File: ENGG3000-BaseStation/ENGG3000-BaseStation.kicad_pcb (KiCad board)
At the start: 4 copper layers, 79 x 43 mm, 57 parts, among them J1 OLED, J10 Cell/Pack 1, J2 Buttons, J3 UltrasonicA, J4 UltrasonicB, J5 USB_C_Receptacle_USB2.0_16P, J7 Power Switch, J8 Cell 3, J9 Cell 2, Q1 SS8050, Q2 AO3401A, SW1 RESET, SW2 BOOT, U1 ESP32-S3-WROOM-1-N16R8, U2 TPS63001DRCR, U3 CN3085

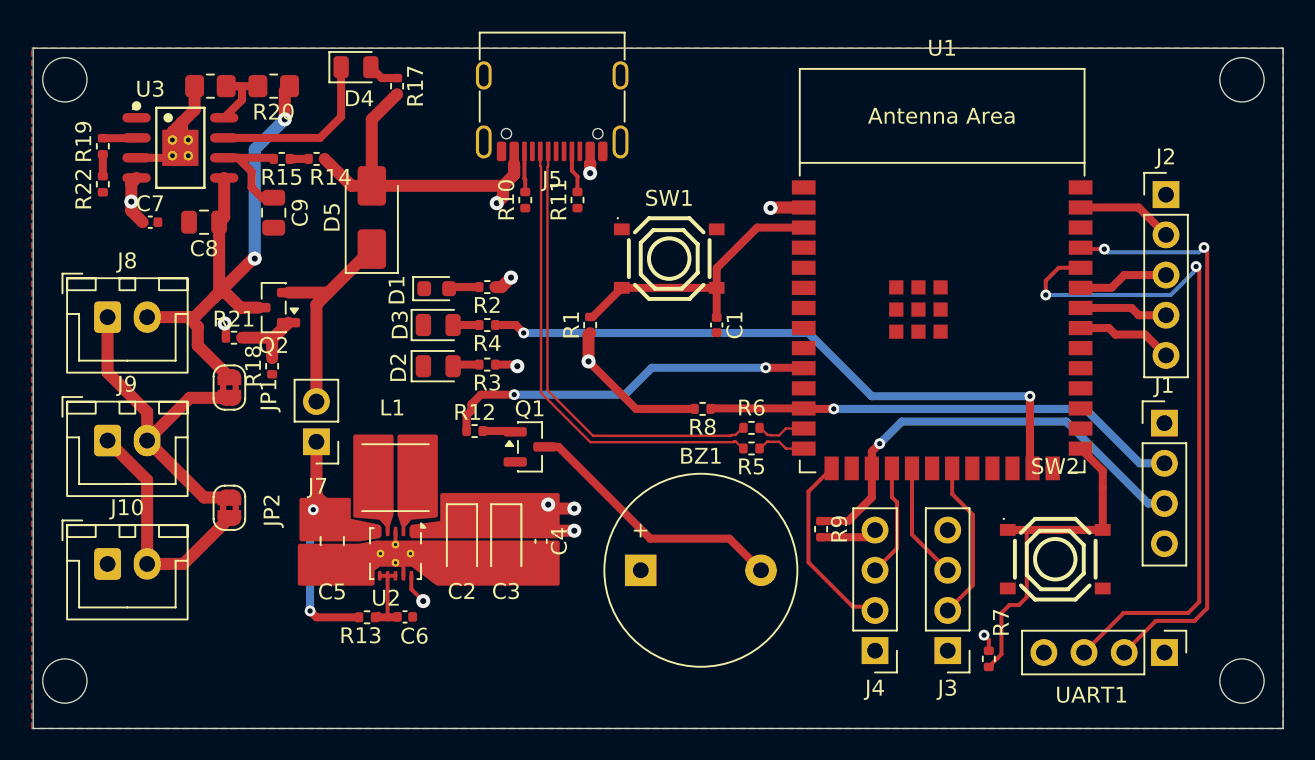
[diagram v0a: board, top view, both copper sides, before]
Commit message: Production ready PCB
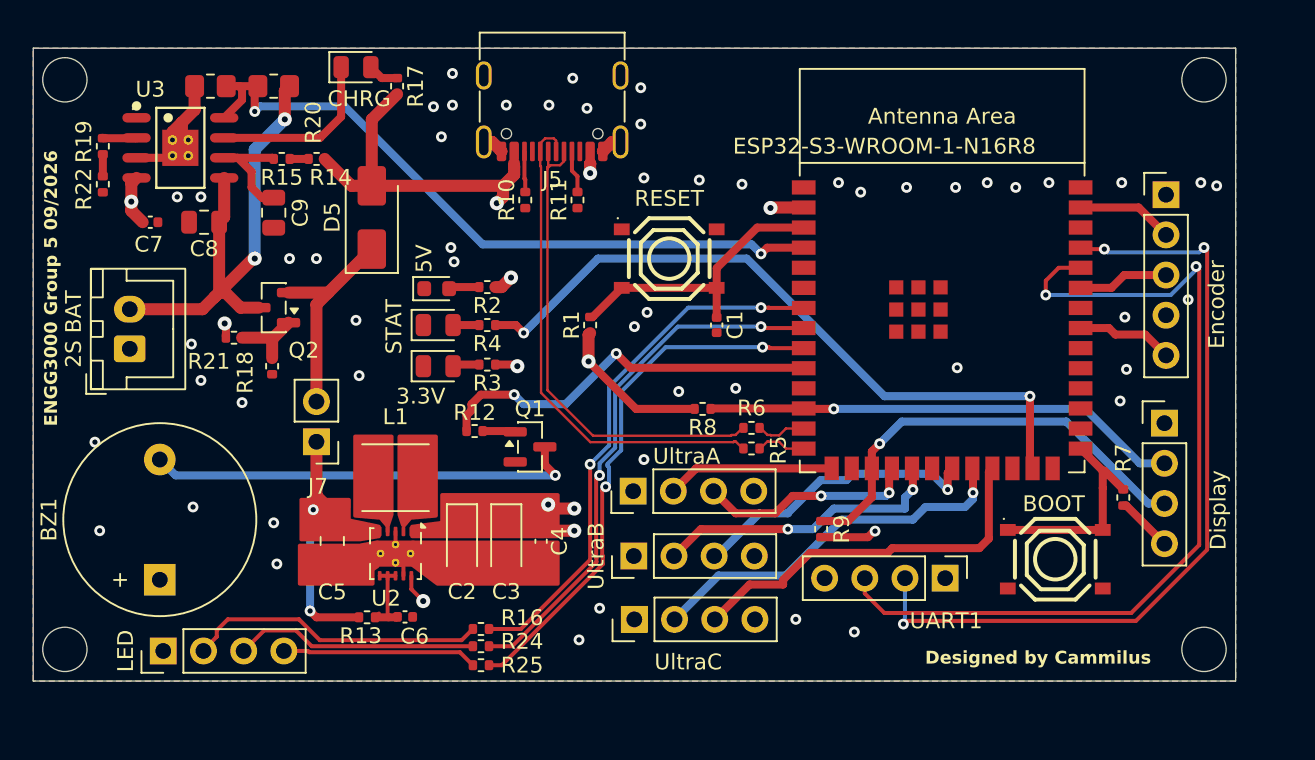
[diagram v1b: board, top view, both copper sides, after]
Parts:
- removed J8: Cell 3, Connector_JST:JST_XH_B2B-XH-A_1x02_P2.50mm_Vertical
- removed J9: Cell 2, Connector_JST:JST_XH_B2B-XH-A_1x02_P2.50mm_Vertical
- removed JP1, JP2: SolderJumper, Jumper:SolderJumper-2_P1.3mm_Bridged2Bar_RoundedPad1.0x1.5mm
- added G***: LOGO, LOGO, B.Cu at (136.5, 79.5)
- added G***: LOGO, LOGO, B.Cu at (167.8, 80.9)
- added LED: RGB LED, Connector_PinHeader_2.54mm:PinHeader_1x04_P2.54mm_Vertical, F.Cu at (118.2, 98.1)
- added R16: 330R, Resistor_SMD:R_0402_1005Metric, F.Cu at (138.3, 96.7)
- added R24: 220R, Resistor_SMD:R_0402_1005Metric, F.Cu at (138.3, 97.8)
- added R25: 220R, Resistor_SMD:R_0402_1005Metric, F.Cu at (138.3, 99.0)
- added UltraC: UltrasonicC, Connector_PinHeader_2.54mm:PinHeader_1x04_P2.54mm_Vertical, F.Cu at (148.0, 96.1)
- 2S BAT: renamed from J10; value Cell/Pack 1 -> NiMH 2S Pack
- Encoder: renamed from J2; value Buttons -> Encoder
- moved BZ1 30.4 mm to (118.0, 93.6), turned to 90 degrees
- moved UltraB 20.7 mm to (148.0, 92.1), turned to 90 degrees
- moved UltraA 18.3 mm to (147.9, 88.0), turned to 90 degrees
- moved UART1 14.6 mm to (167.6, 93.5)
- moved 2S BAT 13.7 mm to (116.1, 79.0), turned to 90 degrees
- moved R7 13.3 mm to (178.9, 88.4), turned to -90 degrees
- renumbered D2 to 3.3V, D1 to 5V, SW2 to BOOT, D4 to CHRG, J1 to Display, U1 to ESP32-S3-WROOM-1-N16R8, SW1 to RESET, D3 to STAT, J4 to UltraA, J3 to UltraB
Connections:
- 2S BAT pad 2: Net-(J10-+) -> BAT
- ESP32-S3-WROOM-1-N16R8 pad 22: unconnected-(U1-GPIO14/TOUCH14/ADC2_CH3/FSPIWP/FSPIDQS/SUBSPIWP-Pad22) -> GPIO14
- ESP32-S3-WROOM-1-N16R8 pad 23: unconnected-(U1-GPIO21-Pad23) -> GPIO21
- ESP32-S3-WROOM-1-N16R8 pad 34: GPIO41 -> unconnected-(U1-MTDI/GPIO41/CLK_OUT1-Pad34)
- ESP32-S3-WROOM-1-N16R8 pad 4: unconnected-(U1-GPIO4/TOUCH4/ADC1_CH3-Pad4) -> FB
- ESP32-S3-WROOM-1-N16R8 pad 7: unconnected-(U1-GPIO7/TOUCH7/ADC1_CH6-Pad7) -> GPIO7
- ESP32-S3-WROOM-1-N16R8 pad 8: unconnected-(U1-GPIO15/U0RTS/ADC2_CH4/XTAL_32K_P-Pad8) -> GPIO15
- ESP32-S3-WROOM-1-N16R8 pad 9: unconnected-(U1-GPIO16/U0CTS/ADC2_CH5/XTAL_32K_N-Pad9) -> GPIO16
- Encoder pad 4: GPIO41 -> GND
- UltraB pad 2: GPIO13 -> GPIO11
- UltraB pad 3: GPIO11 -> GPIO13
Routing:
- net FB: track 4.55 -> 45.1 mm, vias 0 -> 2
- net GPIO16: track 0.00 -> 34.1 mm, vias 0 -> 2
- net GPIO7: track 0.00 -> 34.0 mm, vias 0 -> 2
- net GPIO15: track 0.00 -> 34.0 mm, vias 0 -> 2
- net GPIO21: track 0.00 -> 24.1 mm
- net GPIO14: track 0.00 -> 24.0 mm, vias 0 -> 1
- net Net-(J8--): track 21.8 -> 0.00 mm
- net +3.3V: track 138.3 -> 157.6 mm
- net Net-(J8-R): track 0.00 -> 19.0 mm
- net Net-(J8-G): track 0.00 -> 15.4 mm
- net Net-(J10-+): track 15.2 -> 0.00 mm
- net Net-(U1-U0TXD/GPIO43/CLK_OUT1): track 37.3 -> 51.3 mm, vias 2 -> 3
- net Net-(J8-B): track 0.00 -> 12.3 mm
- net Net-(U1-U0RXD/GPIO44/CLK_OUT2): track 43.7 -> 55.9 mm
- net GPIO11: track 7.37 -> 18.6 mm, vias 0 -> 2
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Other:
- board size 79 x 43 mm -> 76 x 40 mm
- board text added: "Designed by Cammilus"
- board text added: "ENGG3000 Group 5 09/2026"
- board text added: "IAIN IS WATCHING YOU!"
